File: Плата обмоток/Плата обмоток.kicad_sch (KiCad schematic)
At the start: 22 parts, among them J1 4900, J10 4900, J11 4900, J12 4900, J13 4900, J14 A1, J15 A2, J16 B1, J17 B2, J18 C1, J19 C2, J2 4900, J3 4900, J4 Conn_01x02, J6 Conn_01x02, J7 Conn_01x02, J8 4900, J8 Conn_02x02_Odd_Even, J9 4900

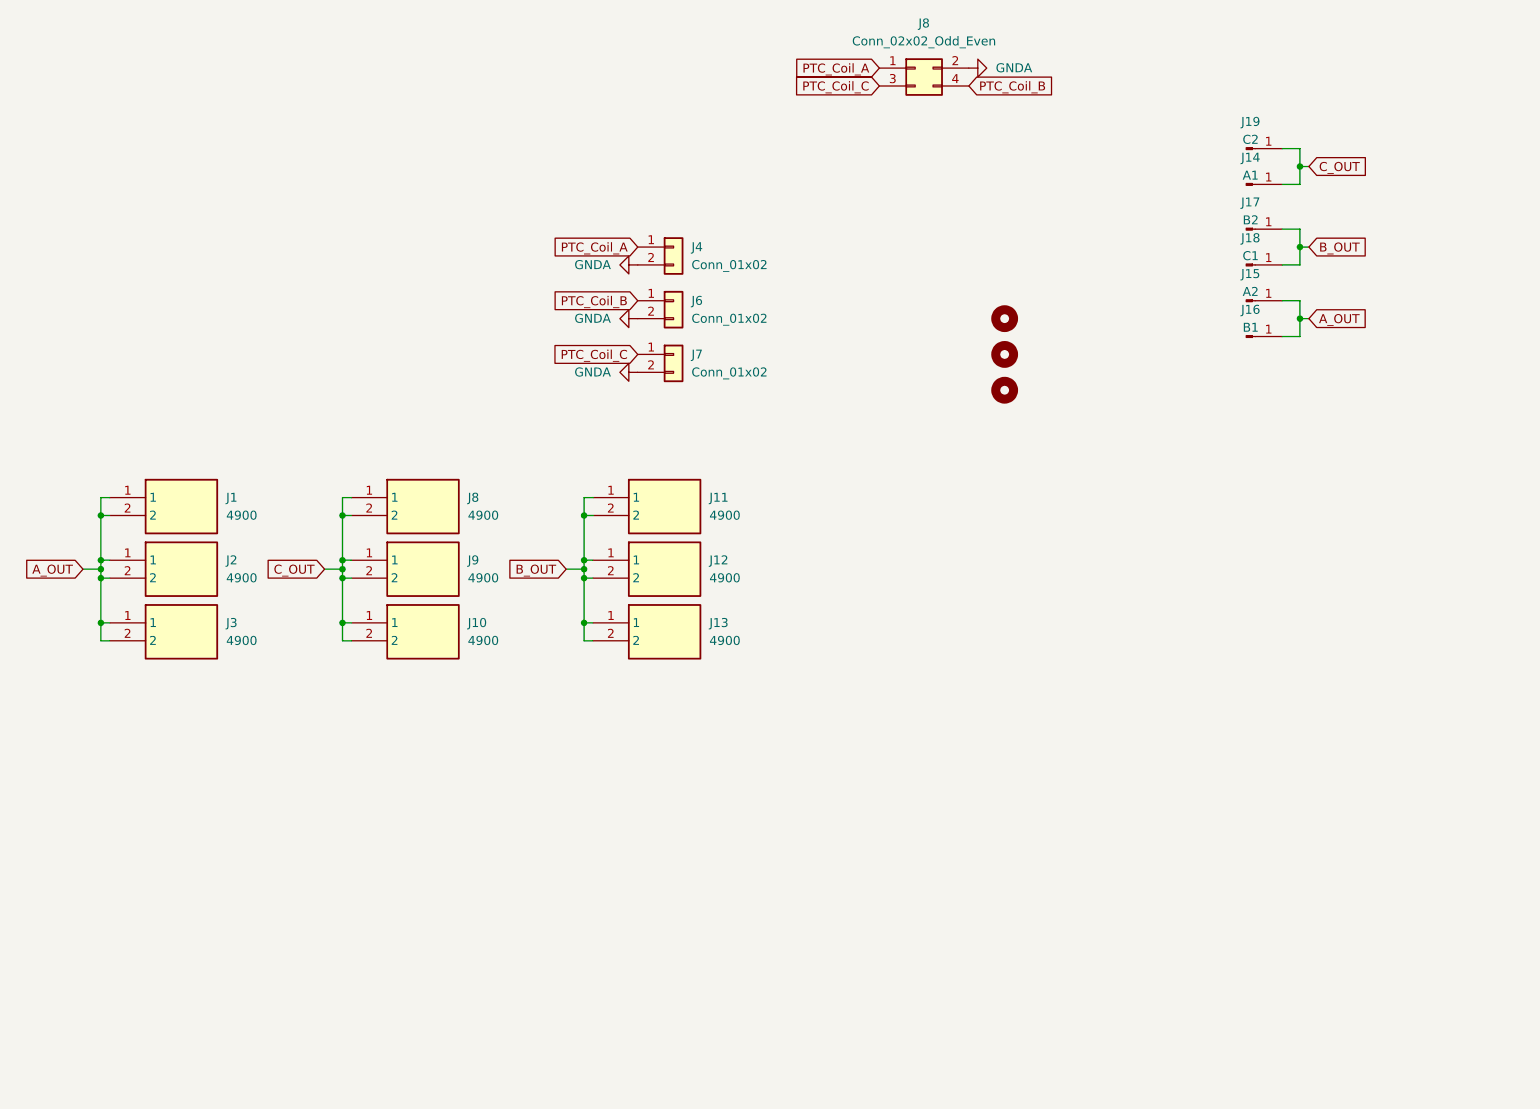
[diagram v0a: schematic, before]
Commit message: Версия под отчётность
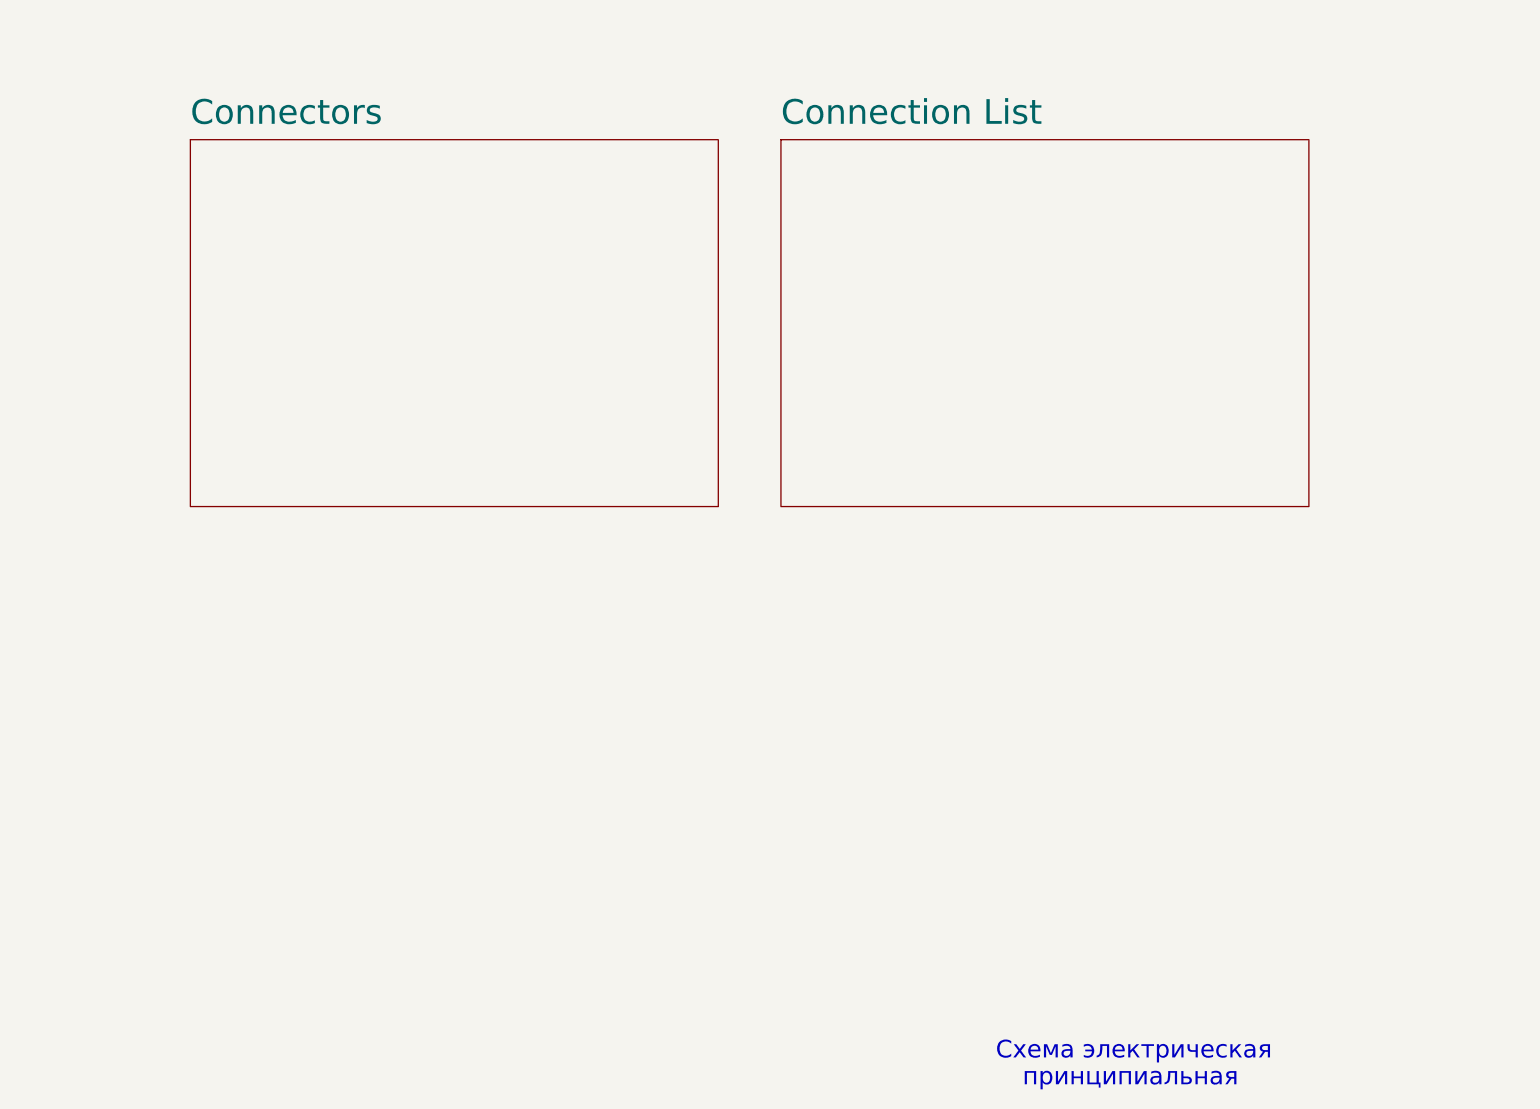
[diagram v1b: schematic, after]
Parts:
- removed H2, H3, H4: MountingHole, MountingHole:MountingHole_3.2mm_M3, symbol Mechanical:MountingHole
- removed J1, J10, J11, J12, J13, J2, J3, J8, J9: 4900, Connector_My:3551, symbol 4900:4900
- removed J14: A1, Connector_My:Coil, symbol Connector:Conn_01x01_Pin
- removed J15: A2, Connector_My:Coil, symbol Connector:Conn_01x01_Pin
- removed J16: B1, Connector_My:Coil, symbol Connector:Conn_01x01_Pin
- removed J17: B2, Connector_My:Coil, symbol Connector:Conn_01x01_Pin
- removed J18: C1, Connector_My:Coil, symbol Connector:Conn_01x01_Pin
- removed J19: C2, Connector_My:Coil, symbol Connector:Conn_01x01_Pin
- removed J4, J6, J7: Conn_01x02, Connector_Molex:Molex_PicoBlade_53048-0210_1x02_P1.25mm_Horizontal, symbol Connector_Generic:Conn_01x02
- removed J8: Conn_02x02_Odd_Even, Connector_PinSocket_2.54mm:PinSocket_2x02_P2.54mm_Vertical, symbol Connector_Generic:Conn_02x02_Odd_Even
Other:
- added sheet Connection List (Connection List.kicad_sch)
- added sheet Connectors (Connectors.kicad_sch)
- note added: "Схема электрическая"
- note added: "принципиальная"
- company: (none) -> Московский Политех
- title: (none) -> Узел соединительный
